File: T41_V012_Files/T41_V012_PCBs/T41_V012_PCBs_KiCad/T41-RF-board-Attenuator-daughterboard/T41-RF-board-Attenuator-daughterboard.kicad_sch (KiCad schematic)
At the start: 6 parts, among them J1 Conn 1, J2 Conn 2, U1 PE4312

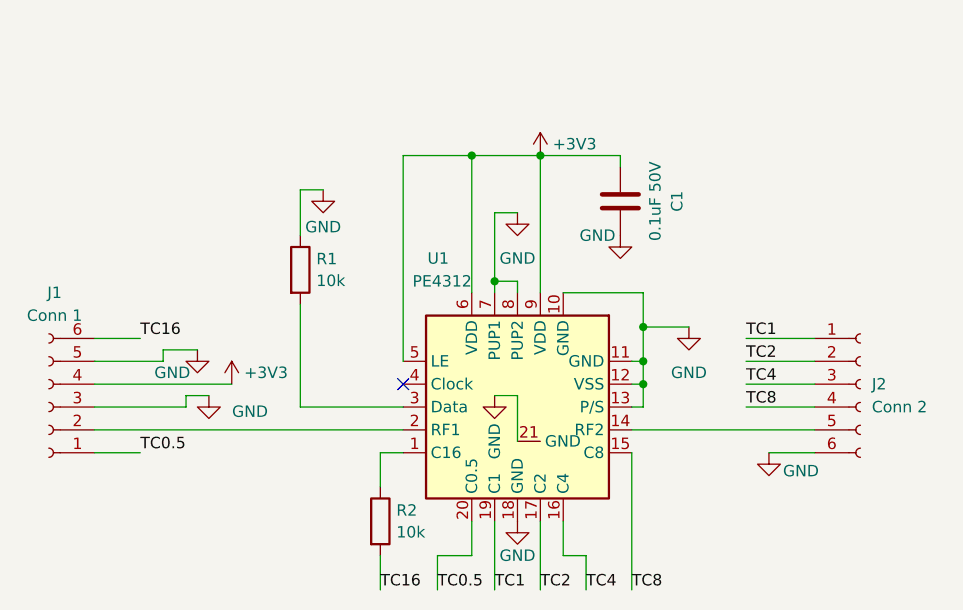
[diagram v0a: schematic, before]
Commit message: New layouts for RF board, clock board, and attenuator board are done
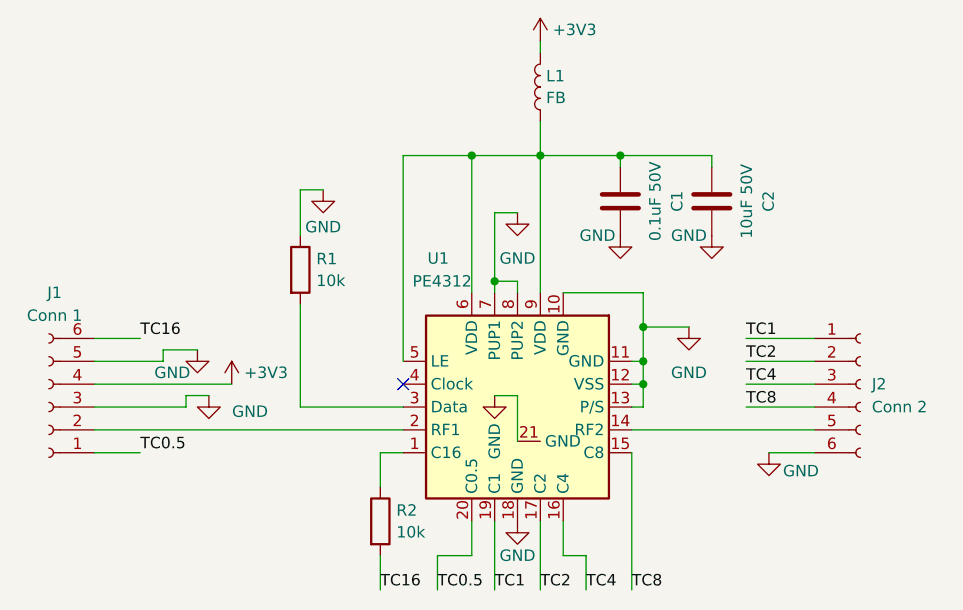
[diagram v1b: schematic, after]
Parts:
- added C2: 10uF 50V, Capacitor_SMD:C_0603_1608Metric, symbol Device:C
- added L1: FB, Resistor_SMD:R_0603_1608Metric, symbol Device:L
- C1: footprint Capacitor_SMD:C_1206_3216Metric -> Capacitor_SMD:C_0603_1608Metric
- R1, R2: footprint Resistor_SMD:R_1206_3216Metric -> Resistor_SMD:R_0603_1608Metric
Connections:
- net +3V3: now also L1.1; no longer C1.2, U1.5 (LE), U1.6 (VDD), U1.9 (VDD)
- net GND: now also C2.1
- new net: C1.2, C2.2, L1.2, U1.5 (LE), U1.6 (VDD), U1.9 (VDD)
